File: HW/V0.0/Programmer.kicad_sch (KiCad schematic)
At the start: 37 parts, among them J4 PG ICSP, Q5 SI2302DS, Q6 SI2302DS, Q7 SI2302DS, SW2 RESET, U5 PIC32MM, U6 SN74LVC1T45, U7 SN74LVC1T45, U8 SN74LVC1T45, U9 SN74LVC1T45

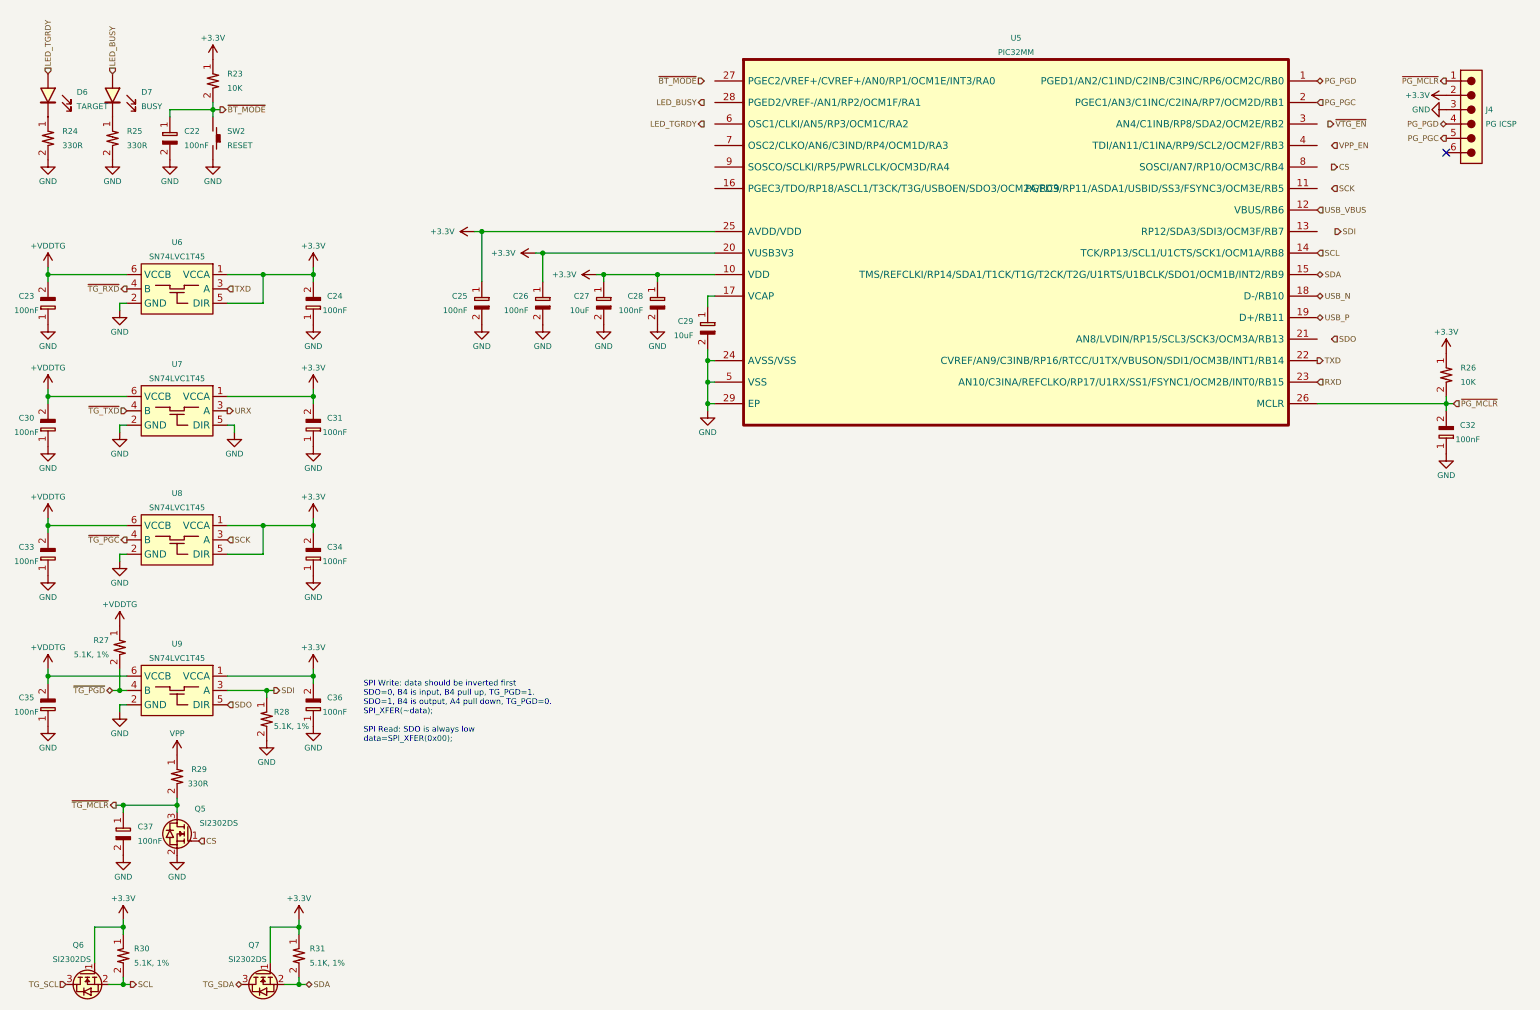
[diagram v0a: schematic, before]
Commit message: PIC16-DevKit-SCH-877 schematic update 6
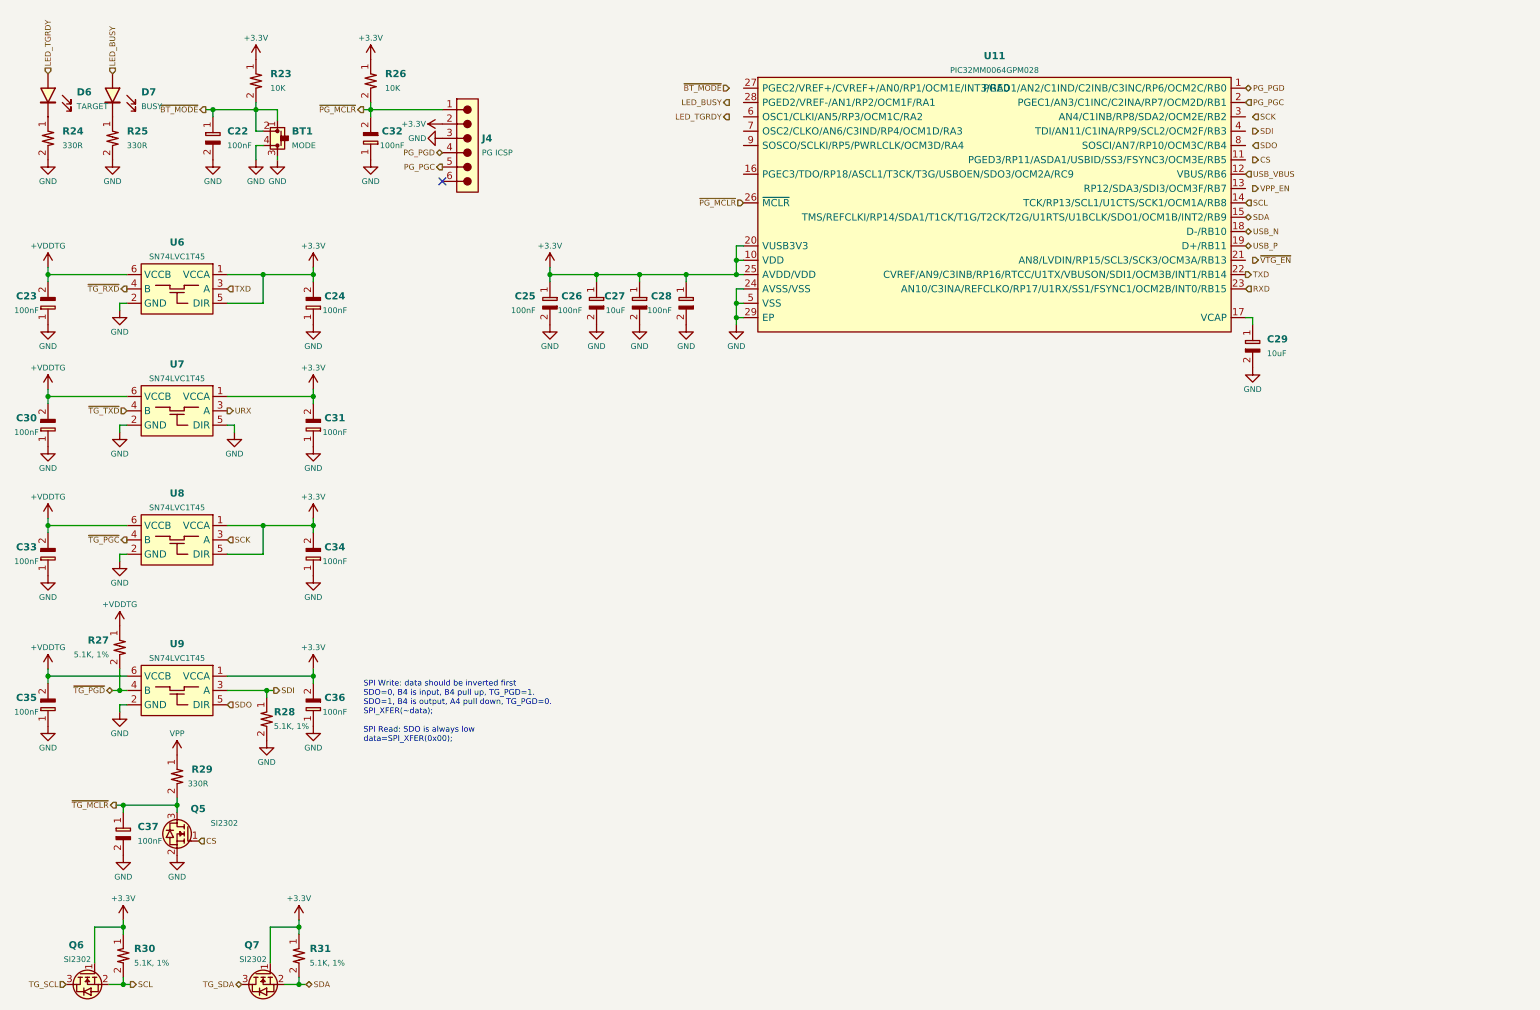
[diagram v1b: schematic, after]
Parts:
- removed SW2: RESET, Triet_KiCAD_Fprint:SW_2P_3.5x6, symbol Triet_KiCAD_Sym:Switch_2P
- removed U5: PIC32MM, Triet_KiCAD_Fprint:UQFN28-EP, symbol Triet_KiCAD_Sym:PIC32MM0064GPM028
- added BT1: MODE, Liem:SW6x6-G, symbol SAMPI:BT2
- added U11: PIC32MM0064GPM028, SAMPI:UQFN28-4x4-EP, symbol SAMPI:PIC32MM0256GPM028-I_M6
- C22, C23, C24, C25, C26, C28, C30, C31, C32, C33, C34, C35, C36, C37: MFT (none) -> Samsung; MNP (none) -> CL10B104KB8NNNC
- C27, C29: MFT (none) -> Samsung; MNP (none) -> CL10A106MQ8NNNC
- D6: MFT (none) -> Harvatek; MNP (none) -> B19Y1NB--20C000113U1930
- D7: MFT (none) -> Harvatek; MNP (none) -> B1911USD-20D000114U1930
- J4: MFT (none) -> DNM; MNP (none) -> NULL; now left out of the parts list
- Q5, Q6, Q7: value SI2302DS -> SI2302; MFT (none) -> Micro Commercial; MNP (none) -> SI2302A-TP
- R23, R26: MFT (none) -> Yageo; MNP (none) -> RC0603JR-0710KL
- R24, R25, R29: MFT (none) -> Yageo; MNP (none) -> RC0603JR-07330RL
- R27, R28, R30, R31: MFT (none) -> Yageo; MNP (none) -> RC0603FR-075K1L
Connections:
- net +3.3V: now also U11.10 (VDD), U11.20 (VUSB3V3), U11.25 (AVDD/VDD)
- net GND: now also BT1.3, BT1.4, U11.24 (AVSS/VSS), U11.29 (EP), U11.5 (VSS)
- net PG_PGC: now also U11.2 (PGEC1/AN3/C1INC/C2INA/RP7/OCM2D/RB1)
- net PG_PGD: now also U11.1 (PGED1/AN2/C1IND/C2INB/C3INC/RP6/OCM2C/RB0)
- net RXD: now also U11.23 (AN10/C3INA/REFCLKO/RP17/U1RX/SS1/FSYNC1/OCM2B/INT0/RB15)
- net SCL: now also U11.14 (TCK/RP13/SCL1/U1CTS/SCK1/OCM1A/RB8)
- net SDA: now also U11.15 (TMS/REFCLKI/RP14/SDA1/T1CK/T1G/T2CK/T2G/U1RTS/U1BCLK/SDO1/OCM1B/INT2/RB9)
- net TXD: now also U11.22 (CVREF/AN9/C3INB/RP16/RTCC/U1TX/VBUSON/SDI1/OCM3B/INT1/RB14)
- net USB_N: now also U11.18 (D-/RB10)
- net USB_P: now also U11.19 (D+/RB11)
- net USB_VBUS: now also U11.12 (VBUS/RB6)
- net ~{BT_MODE}: now also BT1.1, BT1.2
- net ~{PG_MCLR}: now also U11.26 (~{MCLR})
- net at C29.1: now also U11.17 (VCAP)
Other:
- moved on the sheet: C22, C25, C26, C27, C28, C29, C32, J4, R23, R26
